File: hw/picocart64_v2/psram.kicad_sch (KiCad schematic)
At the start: 19 parts, among them U1 LY68L6400SLIT, U2 LY68L6400SLIT, U3 LY68L6400SLIT, U4 LY68L6400SLIT, U5 LY68L6400SLIT, U6 LY68L6400SLIT, U7 LY68L6400SLIT, U8 LY68L6400SLIT, U9 SN74LVC138AQDRQ1

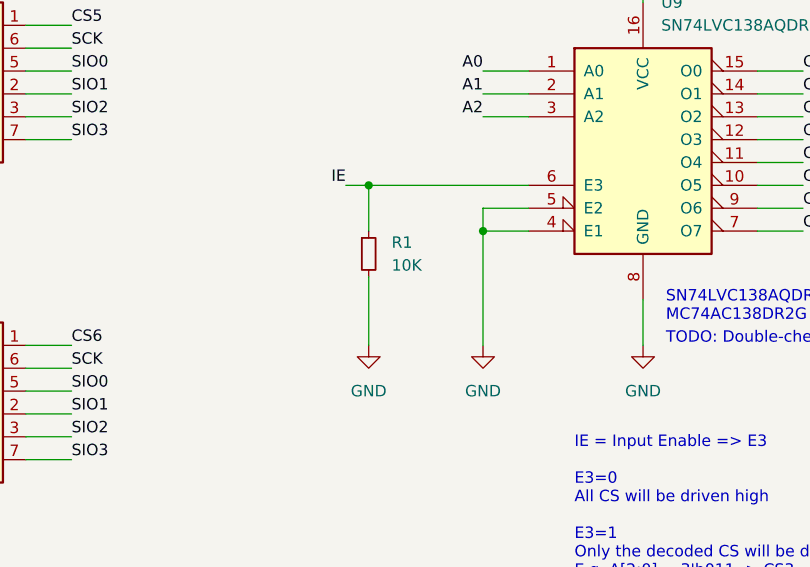
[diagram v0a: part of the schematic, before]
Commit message: hw: Routing progress
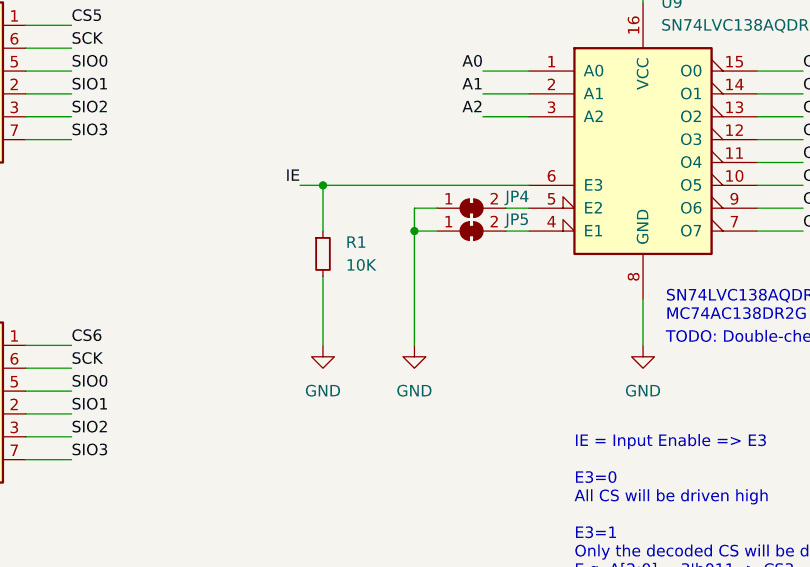
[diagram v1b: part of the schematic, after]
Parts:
- added JP4, JP5: SolderJumper_2_Bridged, picocart64:SolderJumper-2_Small_Closed, symbol Jumper:SolderJumper_2_Bridged
- C1, C2, C3, C4, C5, C6, C7, C8, C9: footprint (none) -> Capacitor_SMD:C_0402_1005Metric
- R1: footprint (none) -> Resistor_SMD:R_0402_1005Metric
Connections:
- net GND: now also JP4.1 (A), JP5.1 (A); no longer U9.4 (E1), U9.5 (E2)
- new net: JP5.2 (B), U9.4 (E1)
- new net: JP4.2 (B), U9.5 (E2)
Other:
- moved on the sheet: R1
